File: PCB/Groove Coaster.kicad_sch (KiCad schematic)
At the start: 17 parts, among them J1 Conn_01x05, J2 Conn_01x05, U1 ProMicro

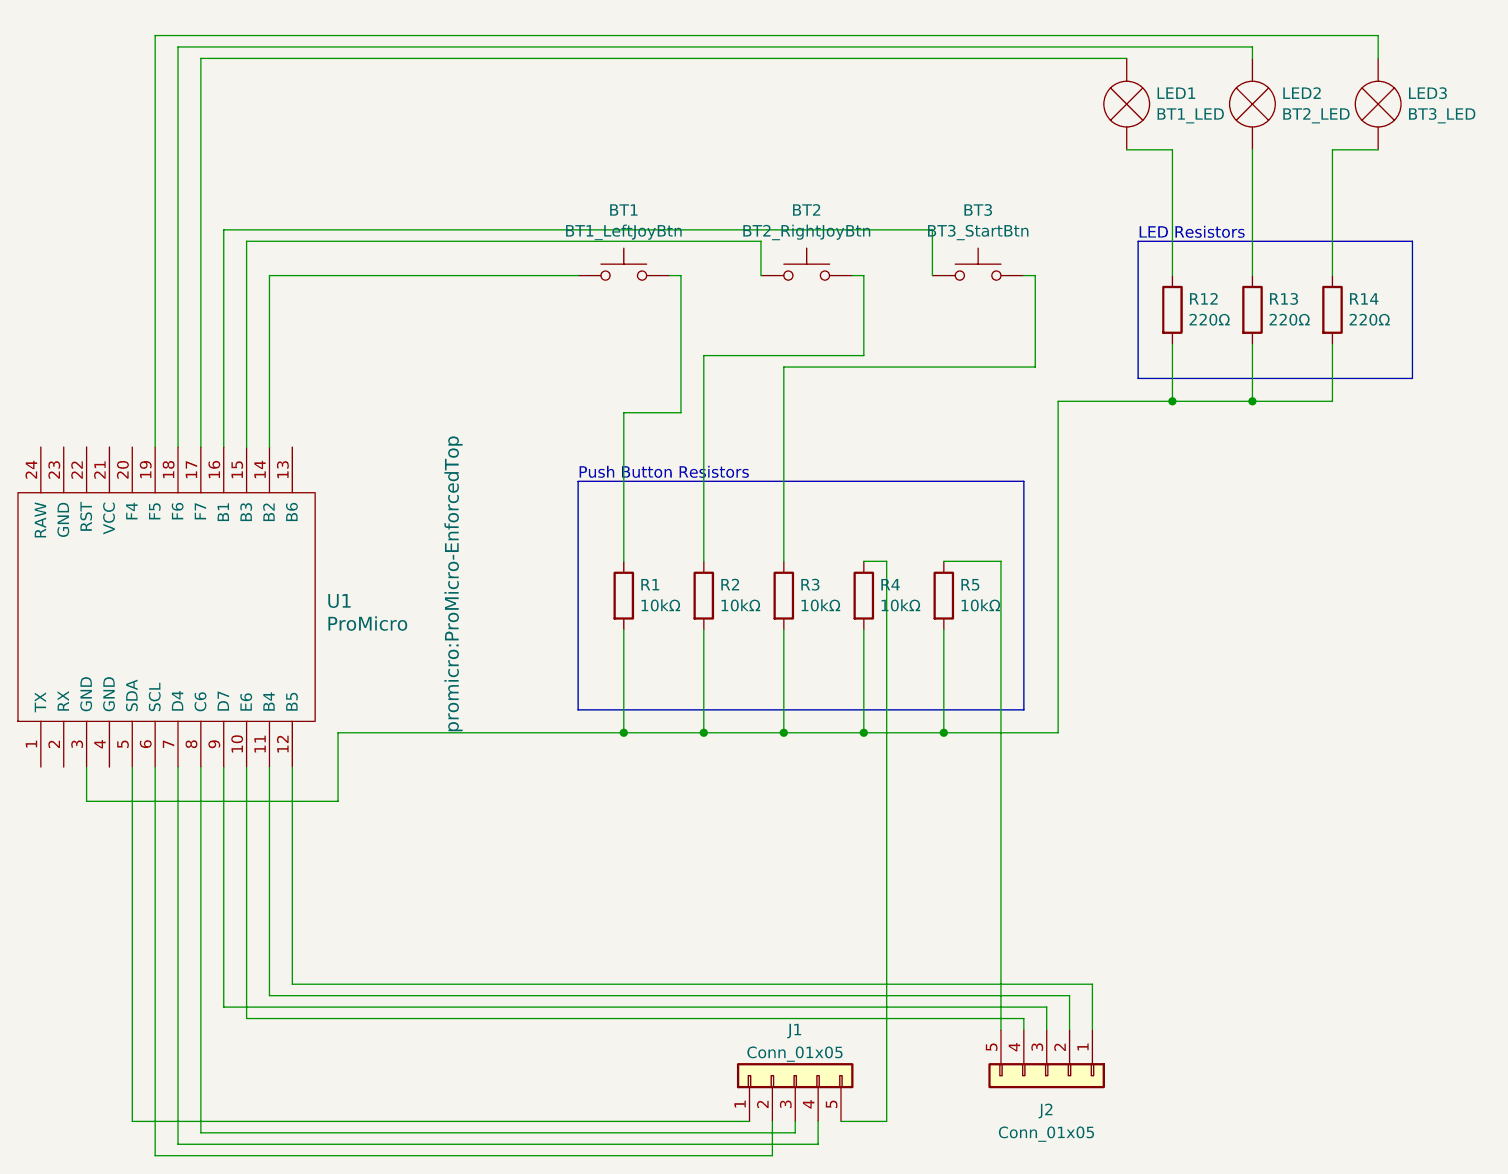
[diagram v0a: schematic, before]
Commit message: oopies
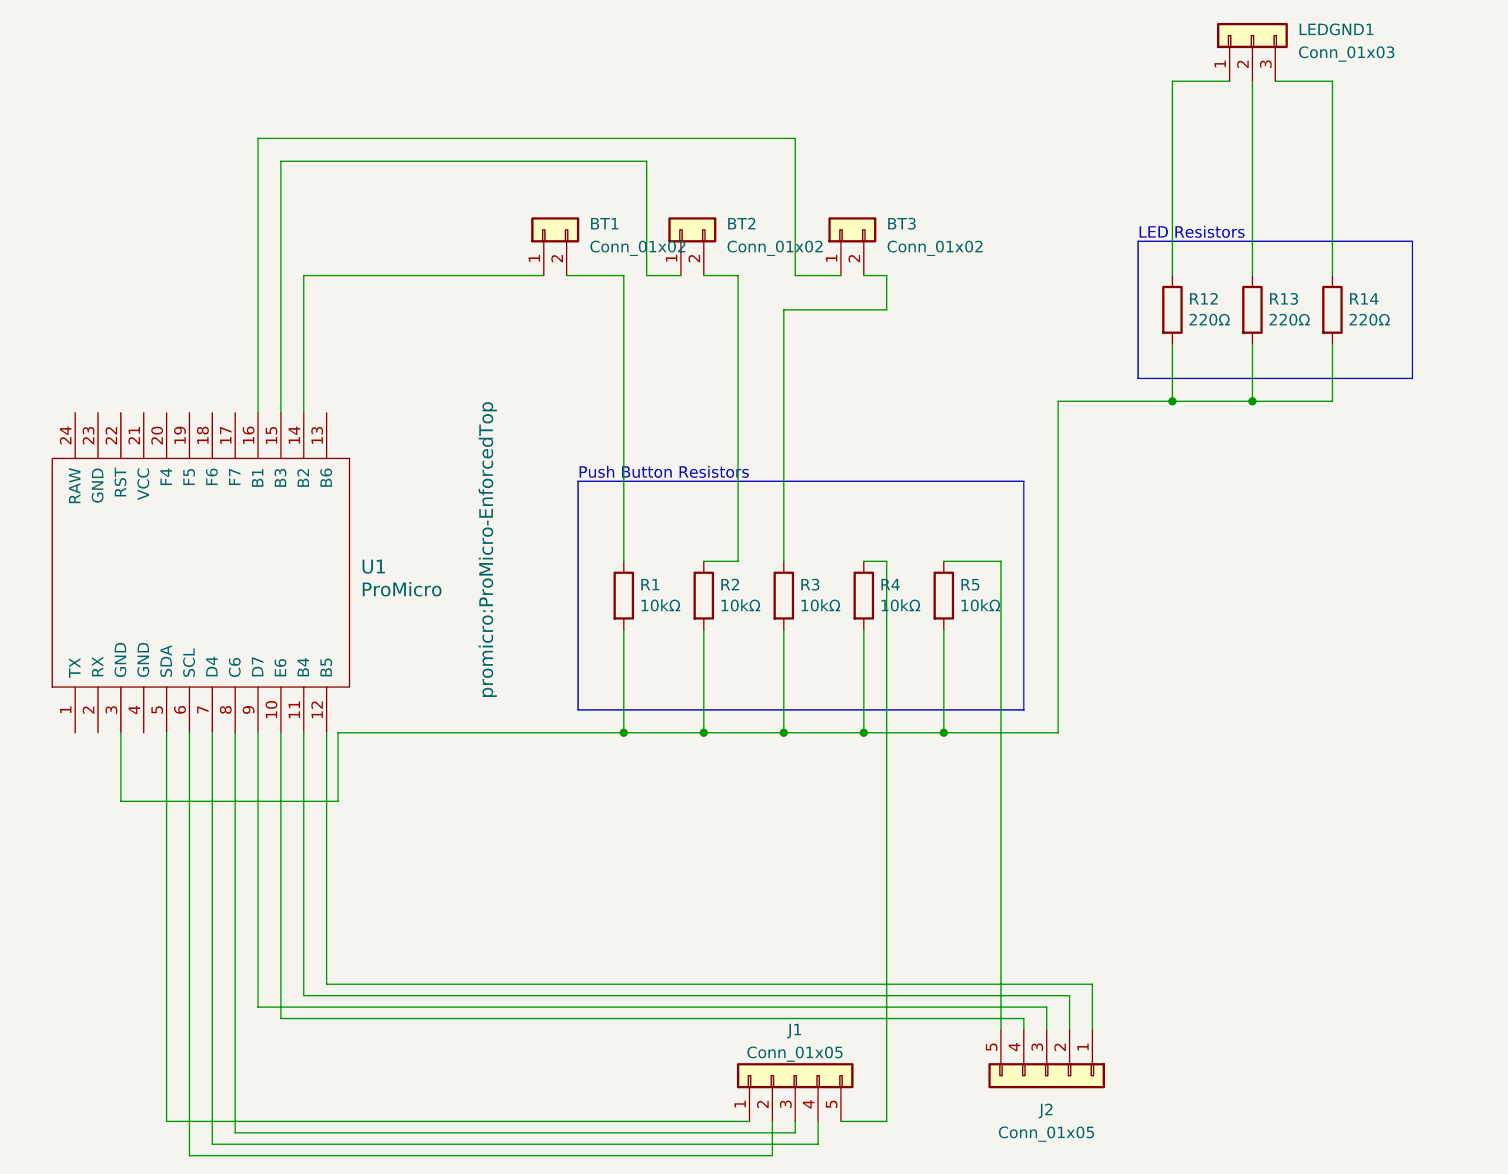
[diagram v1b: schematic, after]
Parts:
- removed BT1: BT1_LeftJoyBtn, Connector_JST:JST_XH_B2B-XH-A_1x02_P2.50mm_Vertical, symbol Switch:SW_Push
- removed BT2: BT2_RightJoyBtn, Connector_JST:JST_XH_B2B-XH-A_1x02_P2.50mm_Vertical, symbol Switch:SW_Push
- removed BT3: BT3_StartBtn, Connector_JST:JST_XH_B2B-XH-A_1x02_P2.50mm_Vertical, symbol Switch:SW_Push
- removed LED1: BT1_LED, Connector_JST:JST_XH_B2B-XH-A_1x02_P2.50mm_Vertical, symbol Device:Lamp
- removed LED2: BT2_LED, Connector_JST:JST_XH_B2B-XH-A_1x02_P2.50mm_Vertical, symbol Device:Lamp
- removed LED3: BT3_LED, Connector_JST:JST_XH_B2B-XH-A_1x02_P2.50mm_Vertical, symbol Device:Lamp
- added BT1, BT2, BT3: Conn_01x02, Connector_JST:JST_XH_B2B-XH-A_1x02_P2.50mm_Vertical, symbol Connector_Generic:Conn_01x02
- added LEDGND1: Conn_01x03, Connector_JST:JST_XH_B3B-XH-A_1x03_P2.50mm_Vertical, symbol Connector_Generic:Conn_01x03
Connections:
- net at R1.1: now also BT1.2 (Pin_2)
- net at R2.1: now also BT2.2 (Pin_2)
- net at R3.1: now also BT3.2 (Pin_2)
- net at R12.1: now also LEDGND1.1 (Pin_1)
- net at R13.1: now also LEDGND1.2 (Pin_2)
- net at R14.1: now also LEDGND1.3 (Pin_3)
- net at U1.14 (B2): now also BT1.1 (Pin_1)
- net at U1.15 (B3): now also BT2.1 (Pin_1)
- net at U1.16 (B1): now also BT3.1 (Pin_1)
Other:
- moved on the sheet: U1
